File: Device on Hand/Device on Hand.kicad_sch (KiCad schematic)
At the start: 14 parts, among them J1 Screw_Terminal_01x02, J2 Screw_Terminal_01x02, J3 Conn_01x15, J4 Screw_Terminal_01x04, U3 SparkFun_SEN-14480_H3LIS331DL, U4 ESP32-DEVKIT-V1

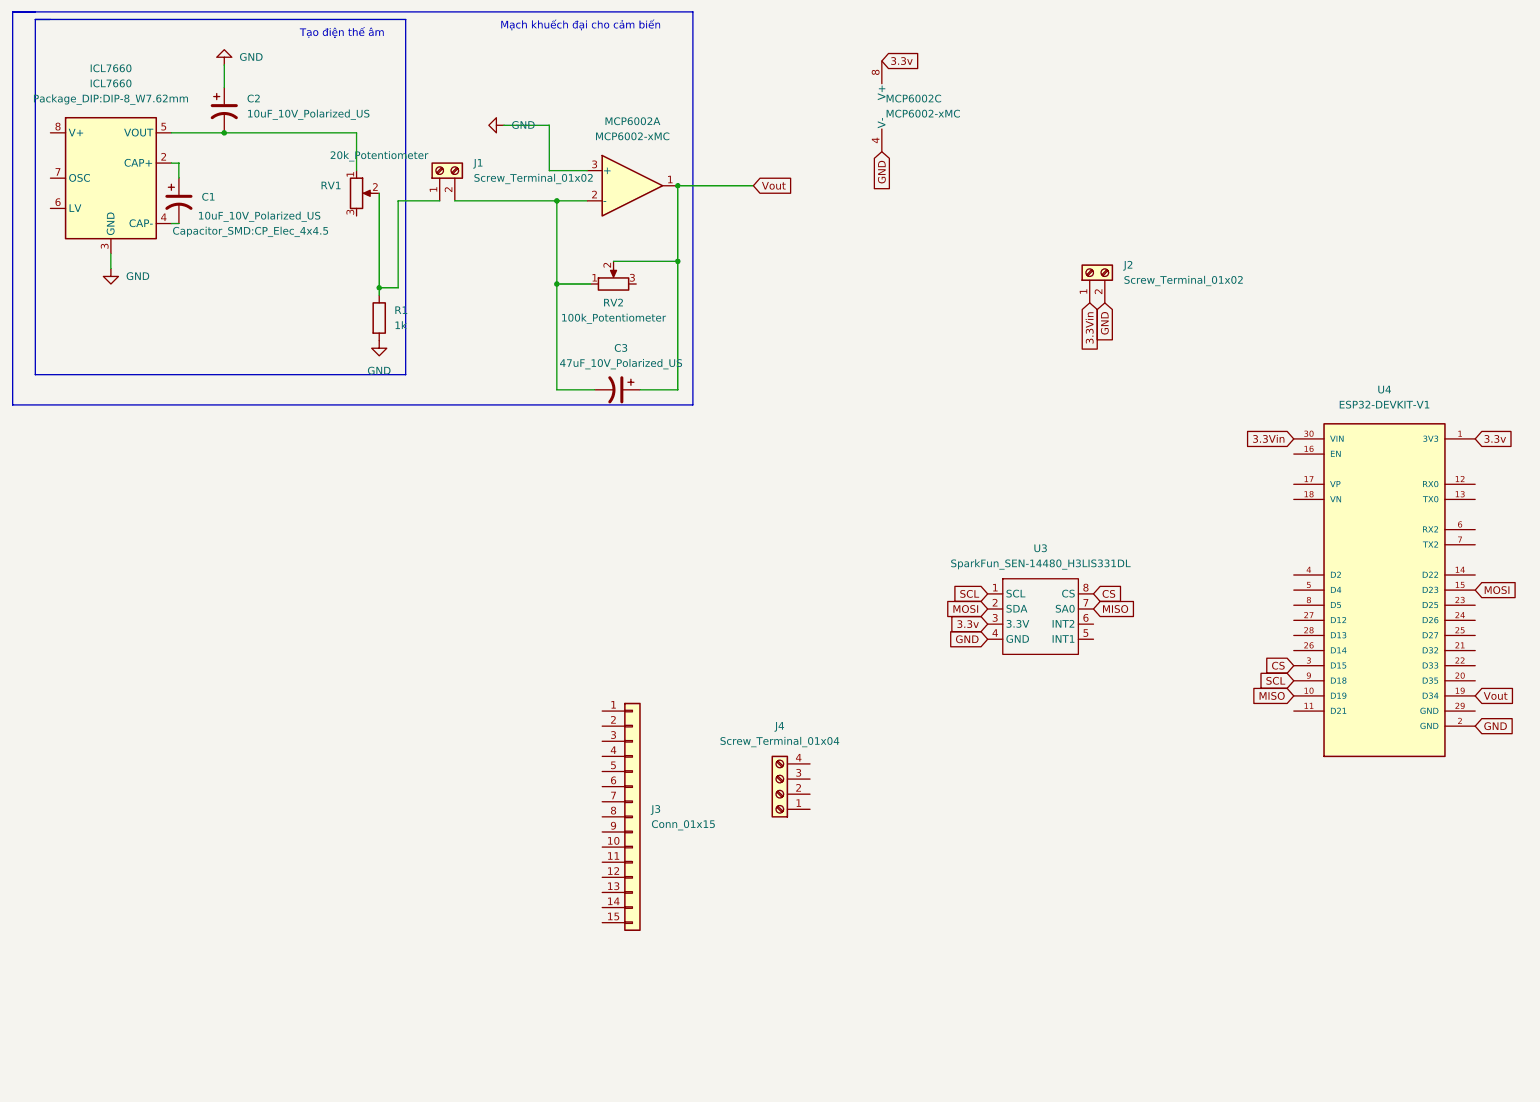
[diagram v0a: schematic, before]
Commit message: update
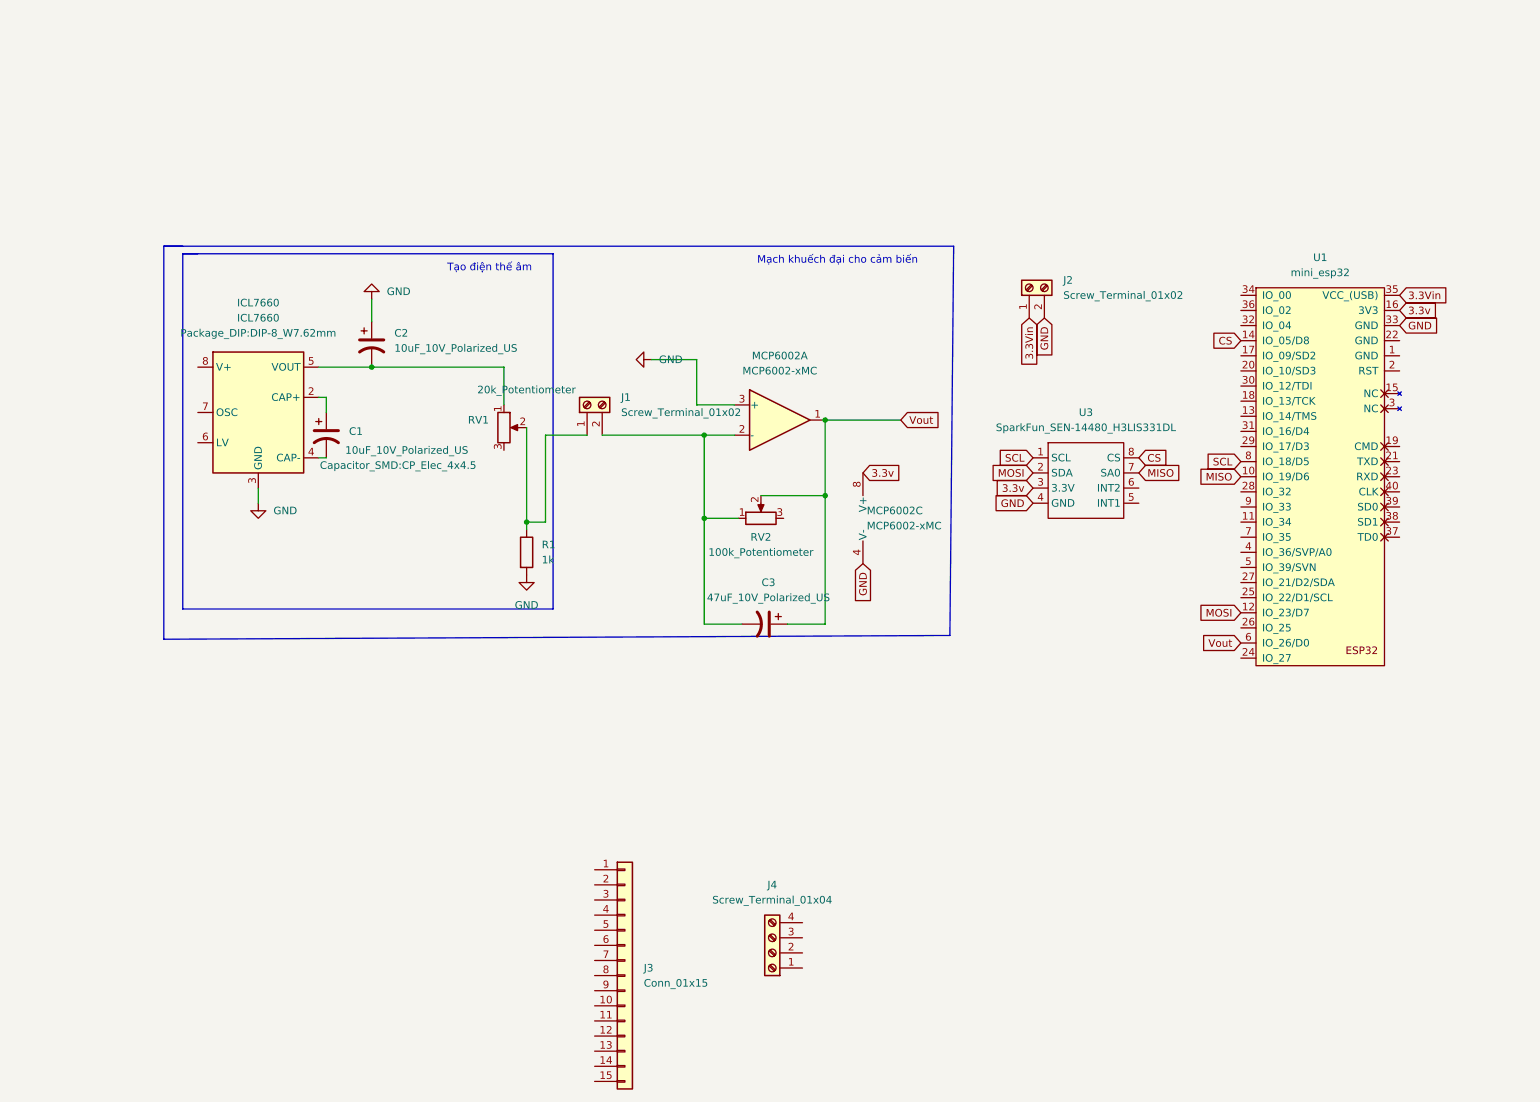
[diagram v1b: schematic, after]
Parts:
- removed U4: ESP32-DEVKIT-V1, ESP32-DEVKIT-V1:MODULE_ESP32_DEVKIT_V1, symbol ESP32-DEVKIT-V1:ESP32-DEVKIT-V1
- added U1: mini_esp32, ESP32_mini:ESP32_mini, symbol ESP32_mini:mini_esp32
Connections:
- net 3.3Vin: now also U1.35 (VCC_(USB))
- net 3.3v: now also U1.16 (3V3)
- net CS: now also U1.14 (IO_05/D8)
- net GND: now also U1.33 (GND)
- net MISO: now also U1.10 (IO_19/D6)
- net MOSI: now also U1.12 (IO_23/D7)
- net SCL: now also U1.8 (IO_18/D5)
- net Vout: now also U1.6 (IO_26/D0)
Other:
- moved on the sheet: C1, C2, C3, ICL7660, J1, J2, J3, J4, MCP6002A, MCP6002C, R1, RV1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
